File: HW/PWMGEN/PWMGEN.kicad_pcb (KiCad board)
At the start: 2 copper layers, 97.8 x 68.6 mm, 33 parts, among them Q1 MMBT3904, U1 STM32F051K8Tx, U2 MCP1825ST-3302E/DB, U3 uA78M05C, U5 LM4132AMF-3.3

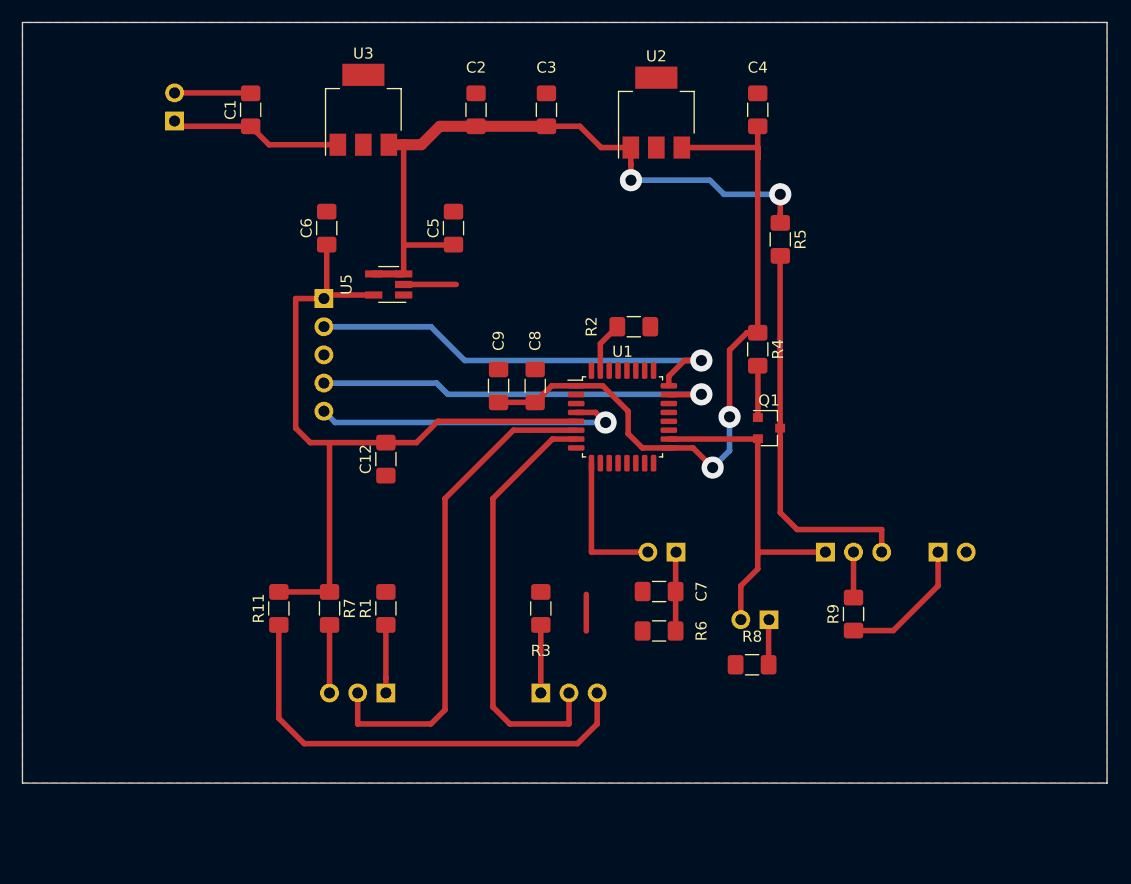
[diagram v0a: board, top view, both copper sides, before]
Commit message: update
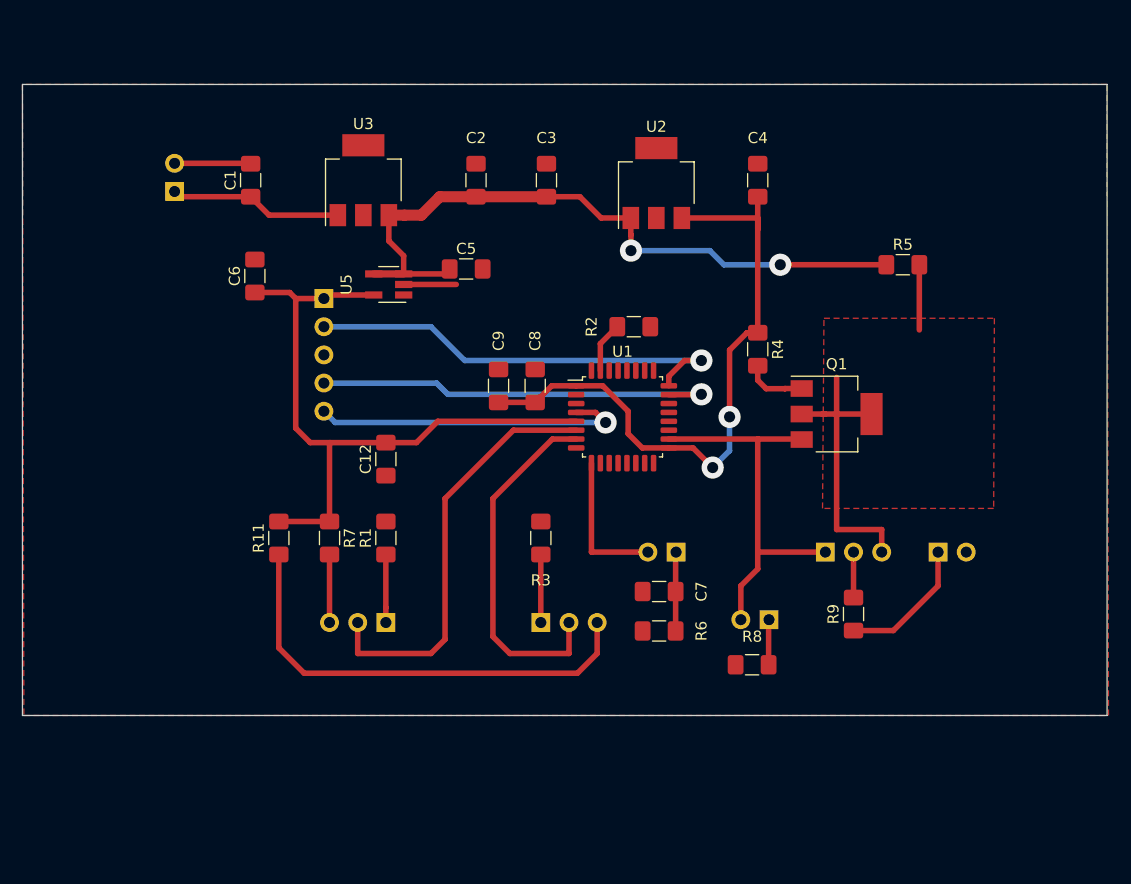
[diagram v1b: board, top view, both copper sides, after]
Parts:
- Q1: value MMBT3904 -> PZT2222A; footprint Package_TO_SOT_SMD:SOT-23 -> Package_TO_SOT_SMD:SOT-223
- moved R5 11.3 mm to (103.5, 39.6), turned to 0 degrees
- moved C6 7.78 mm to (45.1, 40.6)
- moved J_PWR1 6.35 mm to (37.8, 33.0)
- moved U2 6.35 mm to (81.3, 32.3)
- moved C1 6.35 mm to (44.7, 32.0)
- moved C2 6.35 mm to (65.0, 32.0)
- moved C3 6.35 mm to (71.4, 32.0)
- moved C4 6.35 mm to (90.4, 32.0)
- moved U3 6.35 mm to (54.9, 32.0)
- moved J_RV_FREQ1 6.35 mm to (56.9, 71.9)
- moved J_RV_PWM1 6.35 mm to (70.9, 71.9)
- moved R1 6.35 mm to (56.9, 64.3)
- moved R11 6.35 mm to (47.2, 64.3)
- moved R3 6.35 mm to (70.9, 64.3)
- moved R7 6.35 mm to (51.8, 64.3)
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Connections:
- Q1 pad 2: /3V3SIG -> /5VSIG
- Q1 pad 3: /5VSIG -> /3V3SIG
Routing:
- net +3.3VA: track 68.3 -> 61.4 mm
- net +3V3: track 65.6 -> 59.2 mm
- net /PWMADJUST: track 38.8 -> 32.5 mm
- net /FREQADJUST: track 44.6 -> 38.3 mm
- net /3V3SIG: track 31.4 -> 35.0 mm
- net GNDS: track 14.9 -> 11.6 mm
- net /5VSIG: track 34.9 -> 32.2 mm
- net +5V: track 61.7 -> 63.0 mm
- net Net-(Q1-Pad1): track 4.65 -> 5.62 mm
- added copper zone on F.Cu, net /5VSIG
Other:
- board size 97.8 x 68.6 mm -> 97.8 x 56.9 mm

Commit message: updates
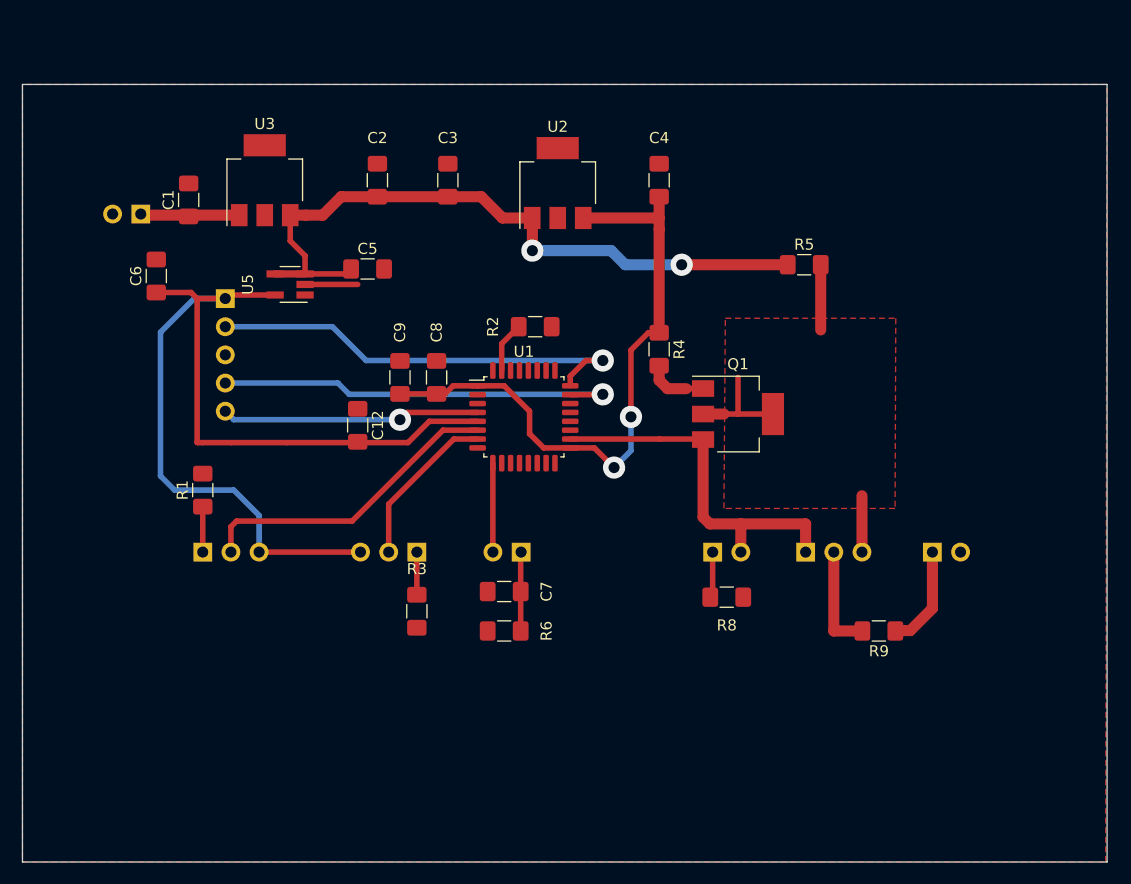
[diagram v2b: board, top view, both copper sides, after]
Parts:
- removed R11, R7: 0R, Resistor_SMD:R_1206_3216Metric_Pad1.42x1.75mm_HandSolder
- moved J_RV_FREQ1 17.7 mm to (40.4, 65.5), turned to 270 degrees
- moved R1 17.1 mm to (40.4, 59.9)
- moved C7 14.0 mm to (67.6, 69.1)
- moved J_SWPSC1 14.0 mm to (69.1, 65.5)
- moved R6 14.0 mm to (67.6, 72.6)
- moved R3 13.0 mm to (59.7, 70.9), turned to 270 degrees
- moved J_RV_PWM1 12.9 mm to (59.7, 65.5), turned to 90 degrees
- moved C8 8.92 mm to (61.5, 49.8)
- moved C9 8.92 mm to (58.2, 49.8)
- moved C5 8.89 mm to (55.2, 40.0)
- moved C2 8.89 mm to (56.1, 32.0)
- moved C4 8.89 mm to (81.5, 32.0)
- moved C6 8.89 mm to (36.2, 40.6)
- moved J_ICSP1 8.89 mm to (42.4, 42.7)
- moved Q1 8.89 mm to (88.6, 53.1)
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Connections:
- J_RV_FREQ1 pad 3: Net-(J_RV_FREQ1-Pad3) -> +3.3VA
- J_RV_PWM1 pad 3: Net-(J_RV_PWM1-Pad3) -> +3.3VA
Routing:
- net Net-(J_RV_PWM1-Pad3): track 41.6 -> 0.00 mm
- net +3.3VA: track 61.4 -> 92.9 mm
- net /PWMADJUST: track 32.5 -> 15.0 mm
- net /5VSIG: track 32.2 -> 20.8 mm
- net /FREQADJUST: track 38.3 -> 28.1 mm
- net GNDS: track 11.6 -> 4.75 mm
- net +9V: track 15.6 -> 8.92 mm
- net Net-(J_RV_FREQ1-Pad3): track 6.13 -> 0.00 mm
- net Net-(LVLSW1-Pad2): track 4.10 -> 9.69 mm
- net /SWRST: track 28.8 -> 23.3 mm
- net /PSC_SELECT: track 13.1 -> 8.01 mm
- net Net-(J_OUT1-Pad1): track 12.3 -> 9.26 mm
- net Net-(J_RV_PWM1-Pad1): track 6.39 -> 3.34 mm
- net Net-(J_RV_FREQ1-Pad1): track 6.13 -> 4.10 mm
- net /3V3SIG: track 35.0 -> 33.6 mm
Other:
- board size 97.8 x 56.9 mm -> 97.8 x 70.1 mm

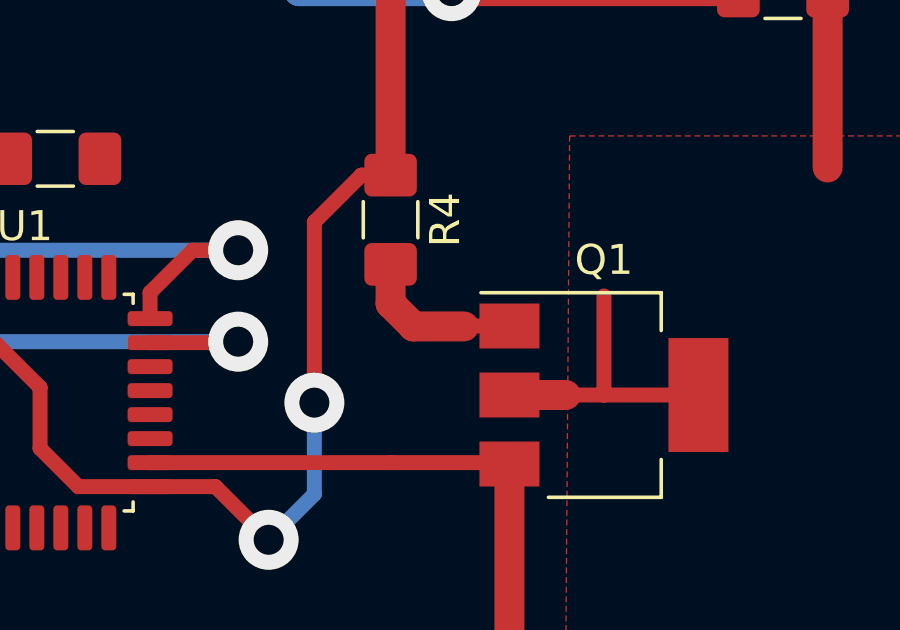
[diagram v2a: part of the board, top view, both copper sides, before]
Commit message: updated sw
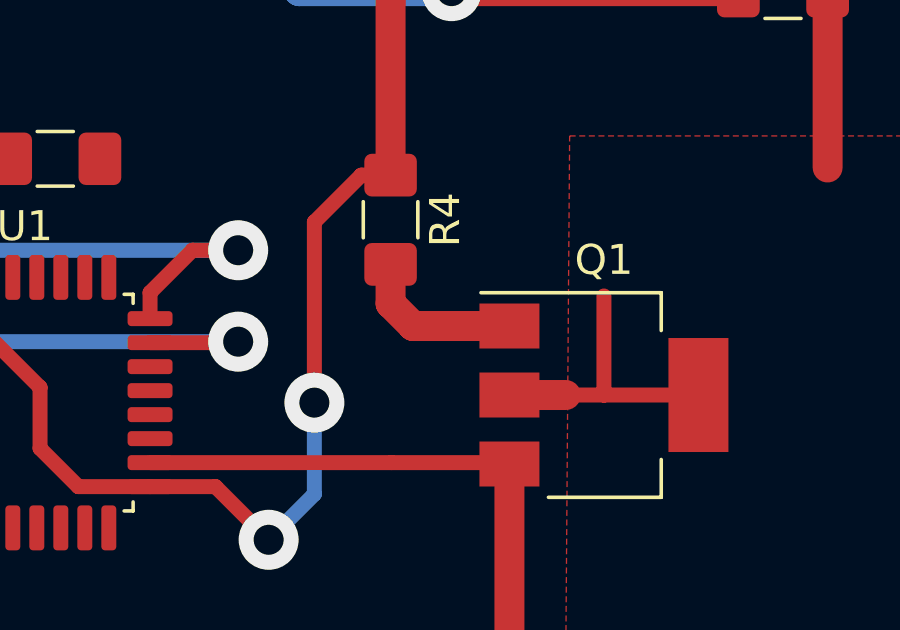
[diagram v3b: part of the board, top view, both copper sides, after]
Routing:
- net Net-(Q1-Pad1): track 5.62 -> 7.13 mm
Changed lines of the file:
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@@
   )
   (setup
-    (last_trace_width 0.5)
+    (last_trace_width 0.25)
     (user_trace_width 0.3)
     (user_trace_width 0.45)
@@
   (segment (start 39.9145 55.6625) (end 40.3495 55.6625) (width 0.5) (layer F.Cu) (net 5))
   (segment (start 40.3495 55.6625) (end 42.9625 55.6625) (width 0.5) (layer F.Cu) (net 5))
+  (segment (start 42.9625 55.6625) (end 47.9695 55.6625) (width 0.5) (layer F.Cu) (net 5))
+  (segment (start 47.9695 55.6625) (end 58.8915 55.6625) (width 0.5) (layer F.Cu) (net 5))
+  (segment (start 45.466 65.532) (end 45.6835 65.7495) (width 0.5) (layer F.Cu) (net 5))
+  (segment (start 45.466 65.532) (end 53.848 65.532) (width 0.5) (layer F.Cu) (net 5))
+  (segment (start 45.466 65.532) (end 45.466 62.23) (width 0.5) (layer B.Cu) (net 5))
+  (segment (start 45.466 62.23) (end 43.18 59.944) (width 0.5) (layer B.Cu) (net 5))
+  (segment (start 43.18 59.944) (end 37.846 59.944) (width 0.5) (layer B.Cu) (net 5))
+  (segment (start 37.846 59.944) (end 36.576 58.674) (width 0.5) (layer B.Cu) (net 5))
+  (segment (start 36.576 58.674) (end 36.576 45.72) (width 0.5) (layer B.Cu) (net 5))
+  (segment (start 39.624 42.672) (end 42.418 42.672) (width 0.5) (layer B.Cu) (net 5))
+  (segment (start 36.576 45.72) (end 39.624 42.672) (width 0.5) (layer B.Cu) (net 5))
   (via (at 58.166 53.594) (size 2) (drill 1) (layers F.Cu B.Cu) (net 6))
   (segment (start 43.18 53.594) (end 42.418 52.832) (width 0.5) (layer B.Cu) (net 6))
@@
   (segment (start 94.742 62.992) (end 94.742 65.532) (width 1) (layer F.Cu) (net 10))
   (segment (start 81.55 48.7885) (end 81.5705 48.768) (width 0.5) (layer F.Cu) (net 11))
-  (segment (start 82.296 50.8) (end 81.534 50.038) (width 1) (layer F.Cu) (net 11))
-  (segment (start 83.982 50.8) (end 82.296 50.8) (width 1) (layer F.Cu) (net 11))
   (segment (start 83.996 50.786) (end 83.982 50.8) (width 0.5) (layer F.Cu) (net 11))
+  (segment (start 85.496 50.786) (end 83.996 50.786) (width 0.5) (layer F.Cu) (net 11))
   (segment (start 81.534 50.038) (end 81.534 48.7315) (width 1) (layer F.Cu) (net 11))
-  (segment (start 85.496 50.786) (end 83.996 50.786) (width 0.5) (layer F.Cu) (net 11))
+  (segment (start 85.496 50.786) (end 82.282 50.786) (width 1) (layer F.Cu) (net 11))
+  (segment (start 82.282 50.786) (end 81.534 50.038) (width 1) (layer F.Cu) (net 11))
   (segment (start 67.342 46.7405) (end 68.8705 45.212) (width 0.5) (layer F.Cu) (net 12))
   (segment (start 67.342 49.165) (end 67.342 46.7405) (width 0.5) (layer F.Cu) (net 12))
+  (segment (start 62.046 54.54) (end 65.167 54.54) (width 0.5) (layer F.Cu) (net 13))
+  (segment (start 53.848 62.738) (end 62.046 54.54) (width 0.5) (layer F.Cu) (net 13))
+  (segment (start 43.434 62.738) (end 53.848 62.738) (width 0.5) (layer F.Cu) (net 13))
+  (segment (start 42.926 65.532) (end 42.926 63.246) (width 0.5) (layer F.Cu) (net 13))
+  (segment (start 42.926 63.246) (end 43.434 62.738) (width 0.5) (layer F.Cu) (net 13))
   (segment (start 65.167 55.34) (end 63.024 55.34) (width 0.5) (layer F.Cu) (net 14))
   (segment (start 63.024 55.34) (end 57.15 61.214) (width 0.5) (layer F.Cu) (net 14))
@@
   (segment (start 102.8335 72.644) (end 102.87 72.6075) (width 0.5) (layer F.Cu) (net 17))
   (segment (start 102.87 72.6075) (end 104.1765 72.6075) (width 1) (layer F.Cu) (net 17))
+  (segment (start 40.386 65.532) (end 40.386 61.4315) (width 0.5) (layer F.Cu) (net 18))
   (segment (start 59.69 66.0035) (end 59.69 69.342) (width 0.5) (layer F.Cu) (net 19))
   (segment (start 69.0515 72.644) (end 69.0515 65.5685) (width 0.5) (layer F.Cu) (net 20))
-  (segment (start 42.9625 55.6625) (end 47.9695 55.6625) (width 0.5) (layer F.Cu) (net 5))
-  (segment (start 47.9695 55.6625) (end 58.8915 55.6625) (width 0.5) (layer F.Cu) (net 5))
-  (segment (start 45.466 65.532) (end 45.6835 65.7495) (width 0.5) (layer F.Cu) (net 5))
-  (segment (start 45.466 65.532) (end 53.848 65.532) (width 0.5) (layer F.Cu) (net 5))
-  (segment (start 45.466 65.532) (end 45.466 62.23) (width 0.5) (layer B.Cu) (net 5))
-  (segment (start 45.466 62.23) (end 43.18 59.944) (width 0.5) (layer B.Cu) (net 5))
-  (segment (start 43.18 59.944) (end 37.846 59.944) (width 0.5) (layer B.Cu) (net 5))
-  (segment (start 37.846 59.944) (end 36.576 58.674) (width 0.5) (layer B.Cu) (net 5))
-  (segment (start 36.576 58.674) (end 36.576 45.72) (width 0.5) (layer B.Cu) (net 5))
-  (segment (start 39.624 42.672) (end 42.418 42.672) (width 0.5) (layer B.Cu) (net 5))
-  (segment (start 36.576 45.72) (end 39.624 42.672) (width 0.5) (layer B.Cu) (net 5))
-  (segment (start 62.046 54.54) (end 65.167 54.54) (width 0.5) (layer F.Cu) (net 13))
-  (segment (start 53.848 62.738) (end 62.046 54.54) (width 0.5) (layer F.Cu) (net 13))
-  (segment (start 43.434 62.738) (end 53.848 62.738) (width 0.5) (layer F.Cu) (net 13))
-  (segment (start 42.926 65.532) (end 42.926 63.246) (width 0.5) (layer F.Cu) (net 13))
-  (segment (start 42.926 63.246) (end 43.434 62.738) (width 0.5) (layer F.Cu) (net 13))
-  (segment (start 40.386 65.532) (end 40.386 61.4315) (width 0.5) (layer F.Cu) (net 18))
   (segment (start 97.282 65.532) (end 97.282 72.644) (width 1) (layer F.Cu) (net 21))
   (segment (start 97.282 72.644) (end 99.8585 72.644) (width 1) (layer F.Cu) (net 21))
